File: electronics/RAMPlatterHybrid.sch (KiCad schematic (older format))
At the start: 57 parts, among them J1 Raspberry_Pi_2_3, J2 Raspberry_Pi_2_3, U1 LM358, U2 74LVC74APW, U3 AV2-8.4-10, U4 AV2-8.4-10, U5 HC4046A, U6 CD74HC4059, U7 AP1117-33, U8 WM8750, U9 NE567

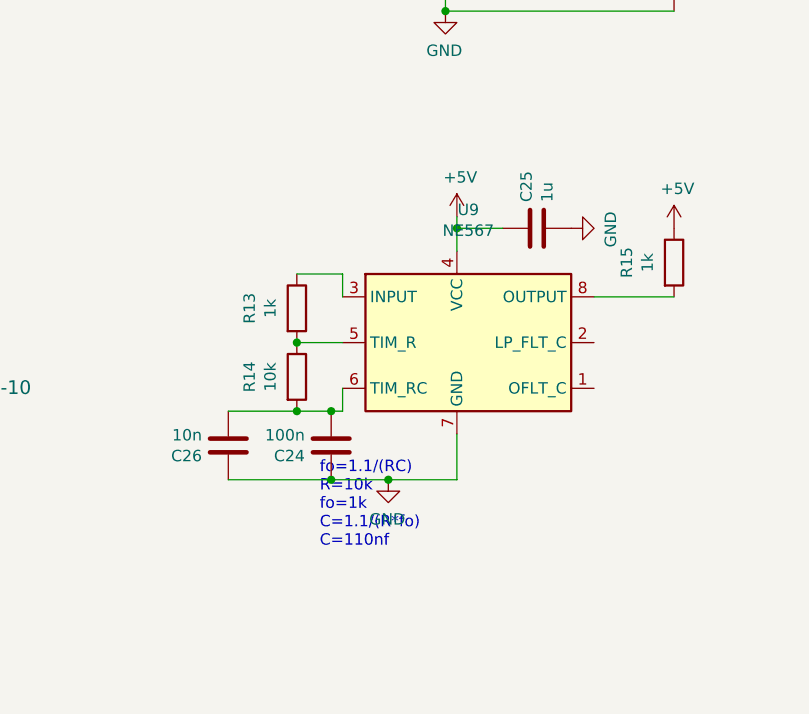
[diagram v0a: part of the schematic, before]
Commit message: added a pdf
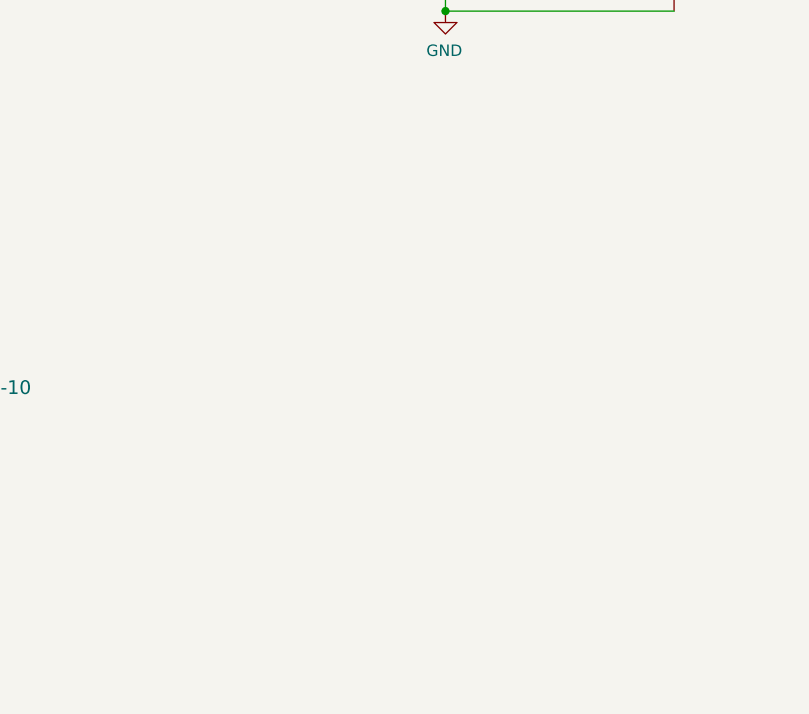
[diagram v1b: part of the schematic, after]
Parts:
- removed C24: 100n, symbol Device:C
- removed C25: 1u, symbol Device:C
- removed C26: 10n, symbol Device:C
- removed R13, R15: 1k, symbol Device:R
- removed R14: 10k, symbol Device:R
- removed U9: NE567, symbol Timer:NE567
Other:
- note removed: "fo=1.1/(RC)\nR=10k\nfo=1k\nC=1.1/(R*fo)\nC=110nf"
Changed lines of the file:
@@
 	10650 3200 10650 3300
-$Comp
-L Timer:NE567 U9
-U 1 1 619FBBE5
-P 9800 5250
-F 0 "U9" H 9850 5831 50  0000 C CNN
-F 1 "NE567" H 9850 5740 50  0000 C CNN
-F 2 "" H 9850 4900 50  0001 L CNN
-F 3 "http://www.ti.com/lit/ds/symlink/lm567.pdf" H 9500 5250 50  0001 C CNN
-	1    9800 5250
-	1    0    0    -1
-$EndComp
-Wire Wire Line
-	9250 5550 9100 5550
-$Comp
-L Device:C C24
-U 1 1 61A0E20C
-P 9250 5700
-F 0 "C24" H 9365 5746 50  0000 L CNN
-F 1 "100n" H 9365 5655 50  0000 L CNN
-F 2 "" H 9288 5550 50  0001 C CNN
-F 3 "~" H 9250 5700 50  0001 C CNN
-	1    9250 5700
-	-1   0    0    1
-$EndComp
-Connection ~ 9250 5850
-Wire Wire Line
-	8800 5850 9250 5850
-Connection ~ 9250 5550
-Wire Wire Line
-	9300 5550 9250 5550
-$Comp
-L Device:C C25
-U 1 1 61A193DE
-P 10150 4750
-F 0 "C25" H 10265 4796 50  0000 L CNN
-F 1 "1u" H 10265 4705 50  0000 L CNN
-F 2 "" H 10188 4600 50  0001 C CNN
-F 3 "~" H 10150 4750 50  0001 C CNN
-	1    10150 4750
-	0    -1   -1   0
-$EndComp
-$Comp
-L Device:R R15
-U 1 1 61A33E22
-P 10750 4900
-F 0 "R15" V 10543 4900 50  0000 C CNN
-F 1 "1k" V 10634 4900 50  0000 C CNN
-F 2 "" V 10680 4900 50  0001 C CNN
-F 3 "~" H 10750 4900 50  0001 C CNN
-	1    10750 4900
-	1    0    0    -1
-$EndComp
-Wire Wire Line
-	9100 5250 9300 5250
-Wire Wire Line
-	9300 5450 9300 5550
-Wire Wire Line
-	9800 5650 9800 5850
-Wire Wire Line
-	9500 5850 9250 5850
-Wire Wire Line
-	9800 5850 9500 5850
-Connection ~ 9500 5850
-$Comp
-L power:GND #PWR0102
-U 1 1 61A16162
-P 9500 5850
-F 0 "#PWR0102" H 9500 5600 50  0001 C CNN
-F 1 "GND" H 9505 5677 50  0000 C CNN
-F 2 "" H 9500 5850 50  0001 C CNN
-F 3 "" H 9500 5850 50  0001 C CNN
-	1    9500 5850
-	-1   0    0    -1
-$EndComp
-$Comp
-L power:+5V #PWR0103
-U 1 1 61A18806
-P 9800 4700
-F 0 "#PWR0103" H 9800 4550 50  0001 C CNN
-F 1 "+5V" H 9815 4873 50  0000 C CNN
-F 2 "" H 9800 4700 50  0001 C CNN
-F 3 "" H 9800 4700 50  0001 C CNN
-	1    9800 4700
-	1    0    0    -1
-$EndComp
-Wire Wire Line
-	10000 4750 9800 4750
-Wire Wire Line
-	9800 4750 9800 4700
-Connection ~ 9800 4750
-Wire Wire Line
-	9800 4850 9800 4750
-$Comp
-L power:GND #PWR0104
-U 1 1 61A295BD
-P 10300 4750
-F 0 "#PWR0104" H 10300 4500 50  0001 C CNN
-F 1 "GND" H 10305 4577 50  0000 C CNN
-F 2 "" H 10300 4750 50  0001 C CNN
-F 3 "" H 10300 4750 50  0001 C CNN
-	1    10300 4750
-	0    -1   1    0
-$EndComp
-Wire Wire Line
-	9300 5050 9300 4950
-Wire Wire Line
-	9300 4950 9100 4950
-Wire Wire Line
-	10750 5050 10400 5050
-$Comp
-L power:+5V #PWR0105
-U 1 1 61A3CC92
-P 10750 4750
-F 0 "#PWR0105" H 10750 4600 50  0001 C CNN
-F 1 "+5V" H 10765 4923 50  0000 C CNN
-F 2 "" H 10750 4750 50  0001 C CNN
-F 3 "" H 10750 4750 50  0001 C CNN
-	1    10750 4750
-	1    0    0    -1
-$EndComp
-Text Notes 9200 6150 0    50   ~ 0
-fo=1.1/(RC)\nR=10k\nfo=1k\nC=1.1/(R*fo)\nC=110nf
-$Comp
-L Device:R R14
-U 1 1 619FFDBB
-P 9100 5400
-F 0 "R14" V 8893 5400 50  0000 C CNN
-F 1 "10k" V 8984 5400 50  0000 C CNN
-F 2 "" V 9030 5400 50  0001 C CNN
-F 3 "~" H 9100 5400 50  0001 C CNN
-	1    9100 5400
-	1    0    0    -1
-$EndComp
-Connection ~ 9100 5550
-Wire Wire Line
-	8800 5550 9100 5550
-Connection ~ 9100 5250
-$Comp
-L Device:R R13
-U 1 1 61A2A6B6
-P 9100 5100
-F 0 "R13" V 8893 5100 50  0000 C CNN
-F 1 "1k" V 8984 5100 50  0000 C CNN
-F 2 "" V 9030 5100 50  0001 C CNN
-F 3 "~" H 9100 5100 50  0001 C CNN
-	1    9100 5100
-	1    0    0    -1
-$EndComp
-$Comp
-L Device:C C26
-U 1 1 61A3FC52
-P 8800 5700
-F 0 "C26" H 8915 5746 50  0000 L CNN
-F 1 "10n" H 8915 5655 50  0000 L CNN
-F 2 "" H 8838 5550 50  0001 C CNN
-F 3 "~" H 8800 5700 50  0001 C CNN
-	1    8800 5700
-	-1   0    0    1
-$EndComp
 $Comp
 L Connector:Raspberry_Pi_2_3 J2
